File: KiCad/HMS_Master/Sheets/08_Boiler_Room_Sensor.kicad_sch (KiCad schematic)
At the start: 2 parts, among them U10 DHT11, U20 BOILER_ROOM_SENSOR_SOCKET

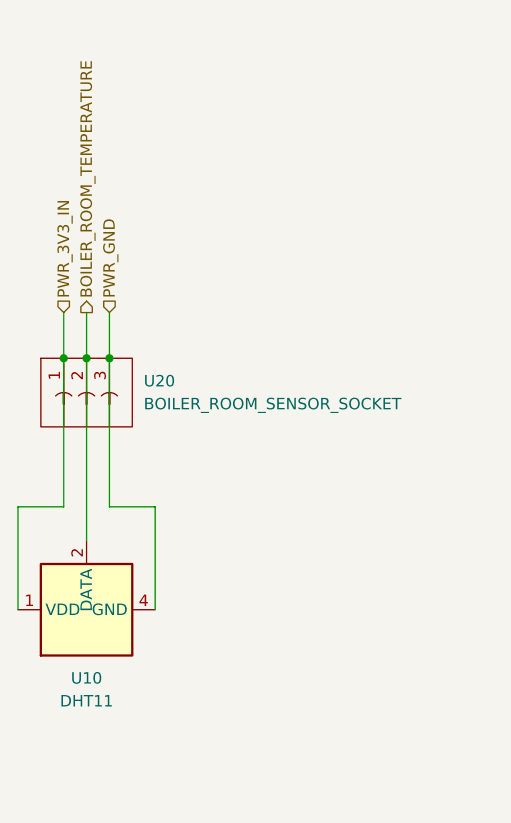
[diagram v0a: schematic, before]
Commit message: Refactor KiCad Master directory structure
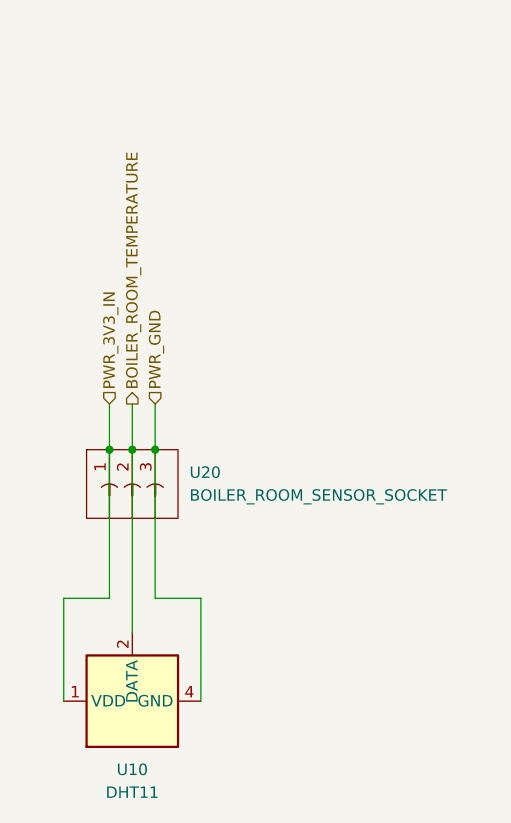
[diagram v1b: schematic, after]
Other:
- moved on the sheet: U10, U20
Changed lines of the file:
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@@
 	(paper "A4")
 	(junction
-		(at 133.35 74.93)
+		(at 138.43 85.09)
 		(diameter 0)
 		(color 255 0 0 1)
 	)
 	(junction
-		(at 135.89 74.93)
+		(at 140.97 85.09)
 		(diameter 0)
 		(color 194 194 194 1)
 	)
 	(junction
-		(at 138.43 74.93)
+		(at 143.51 85.09)
 		(diameter 0)
 		(color 0 0 0 1)
@@
 	(wire
 		(pts
-			(xy 133.35 69.85) (xy 133.35 74.93)
-		)
-		(stroke
-			(width 0.254)
-			(type default)
-			(color 255 0 0 1)
-		)
-	)
-	(wire
-		(pts
-			(xy 128.27 91.44) (xy 128.27 102.87)
-		)
-		(stroke
-			(width 0.254)
-			(type default)
-			(color 255 0 0 1)
-		)
-	)
-	(wire
-		(pts
-			(xy 138.43 91.44) (xy 143.51 91.44)
-		)
-		(stroke
-			(width 0.254)
-			(type default)
-			(color 0 0 0 1)
-		)
-	)
-	(wire
-		(pts
-			(xy 143.51 91.44) (xy 143.51 102.87)
-		)
-		(stroke
-			(width 0.254)
-			(type default)
-			(color 0 0 0 1)
-		)
-	)
-	(wire
-		(pts
-			(xy 135.89 69.85) (xy 135.89 74.93)
+			(xy 138.43 80.01) (xy 138.43 85.09)
+		)
+		(stroke
+			(width 0.254)
+			(type default)
+			(color 255 0 0 1)
+		)
+	)
+	(wire
+		(pts
+			(xy 133.35 101.6) (xy 133.35 113.03)
+		)
+		(stroke
+			(width 0.254)
+			(type default)
+			(color 255 0 0 1)
+		)
+	)
+	(wire
+		(pts
+			(xy 143.51 101.6) (xy 148.59 101.6)
+		)
+		(stroke
+			(width 0.254)
+			(type default)
+			(color 0 0 0 1)
+		)
+	)
+	(wire
+		(pts
+			(xy 148.59 101.6) (xy 148.59 113.03)
+		)
+		(stroke
+			(width 0.254)
+			(type default)
+			(color 0 0 0 1)
+		)
+	)
+	(wire
+		(pts
+			(xy 140.97 80.01) (xy 140.97 85.09)
 		)
 		(stroke
@@
 	(wire
 		(pts
-			(xy 133.35 91.44) (xy 128.27 91.44)
-		)
-		(stroke
-			(width 0.254)
-			(type default)
-			(color 255 0 0 1)
-		)
-	)
-	(wire
-		(pts
-			(xy 138.43 74.93) (xy 138.43 91.44)
-		)
-		(stroke
-			(width 0.254)
-			(type default)
-			(color 0 0 0 1)
-		)
-	)
-	(wire
-		(pts
-			(xy 138.43 69.85) (xy 138.43 74.93)
-		)
-		(stroke
-			(width 0.254)
-			(type default)
-			(color 0 0 0 1)
-		)
-	)
-	(wire
-		(pts
-			(xy 135.89 74.93) (xy 135.89 95.25)
+			(xy 138.43 101.6) (xy 133.35 101.6)
+		)
+		(stroke
+			(width 0.254)
+			(type default)
+			(color 255 0 0 1)
+		)
+	)
+	(wire
+		(pts
+			(xy 143.51 85.09) (xy 143.51 101.6)
+		)
+		(stroke
+			(width 0.254)
+			(type default)
+			(color 0 0 0 1)
+		)
+	)
+	(wire
+		(pts
+			(xy 143.51 80.01) (xy 143.51 85.09)
+		)
+		(stroke
+			(width 0.254)
+			(type default)
+			(color 0 0 0 1)
+		)
+	)
+	(wire
+		(pts
+			(xy 140.97 85.09) (xy 140.97 105.41)
 		)
 		(stroke
@@
 	(wire
 		(pts
-			(xy 133.35 74.93) (xy 133.35 91.44)
+			(xy 138.43 85.09) (xy 138.43 101.6)
 		)
 		(stroke
@@
 	(hierarchical_label "PWR_GND"
 		(shape input)
-		(at 138.43 69.85 90)
+		(at 143.51 80.01 90)
 		(effects
 			(font
@@
 	(hierarchical_label "BOILER_ROOM_TEMPERATURE"
 		(shape output)
-		(at 135.89 69.85 90)
+		(at 140.97 80.01 90)
 		(effects
 			(font
@@
 	(hierarchical_label "PWR_3V3_IN"
 		(shape input)
-		(at 133.35 69.85 90)
+		(at 138.43 80.01 90)
 		(effects
 			(font
@@
 	(symbol
 		(lib_id "HMS_Symbols:CONN_JST_PH_3P")
-		(at 135.89 78.74 0)
+		(at 140.97 88.9 0)
 		(unit 1)
 		(body_style 1)
@@
 		(fields_autoplaced yes)
 		(property "Reference" "U20"
-			(at 142.24 77.4699 0)
+			(at 147.32 87.6299 0)
 			(show_name no)
 			(do_not_autoplace no)
@@
 		)
 		(property "Value" "BOILER_ROOM_SENSOR_SOCKET"
-			(at 142.24 80.0099 0)
+			(at 147.32 90.1699 0)
 			(show_name no)
 			(do_not_autoplace no)
@@
 		)
 		(property "Footprint" "Connector_JST:JST_XH_B3B-XH-A_1x03_P2.50mm_Vertical"
-			(at 135.89 85.852 0)
+			(at 140.97 96.012 0)
 			(hide yes)
 			(show_name no)
@@
 		)
 		(property "Datasheet" ""
-			(at 135.89 78.74 0)
+			(at 140.97 88.9 0)
 			(hide yes)
 			(show_name no)
@@
 		)
 		(property "Description" ""
-			(at 135.89 78.74 0)
+			(at 140.97 88.9 0)
 			(hide yes)
 			(show_name no)
@@
 	(symbol
 		(lib_id "Sensor:DHT11")
-		(at 135.89 102.87 90)
+		(at 140.97 113.03 90)
 		(unit 1)
 		(body_style 1)
@@
 		(fields_autoplaced yes)
 		(property "Reference" "U10"
-			(at 135.89 110.49 90)
+			(at 140.97 120.65 90)
 			(show_name no)
 			(do_not_autoplace no)
@@
 		)
 		(property "Value" "DHT11"
-			(at 135.89 113.03 90)
+			(at 140.97 123.19 90)
 			(show_name no)
 			(do_not_autoplace no)
@@
 		)
 		(property "Footprint" "Sensor:Aosong_DHT11_5.5x12.0_P2.54mm"
-			(at 146.05 102.87 0)
+			(at 151.13 113.03 0)
 			(hide yes)
 			(show_name no)
@@
 		)
 		(property "Datasheet" "http://akizukidenshi.com/download/ds/aosong/DHT11.pdf"
-			(at 129.54 99.06 0)
+			(at 134.62 109.22 0)
 			(hide yes)
 			(show_name no)
@@
 		)
 		(property "Description" "3.3V to 5.5V, temperature and humidity module, DHT11"
-			(at 135.89 102.87 0)
-			(hide yes)
-			(show_name no)
+			(at 140.97 113.03 0)
+			(hide yes)
+			(show_name no)
